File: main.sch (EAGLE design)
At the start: 3 parts

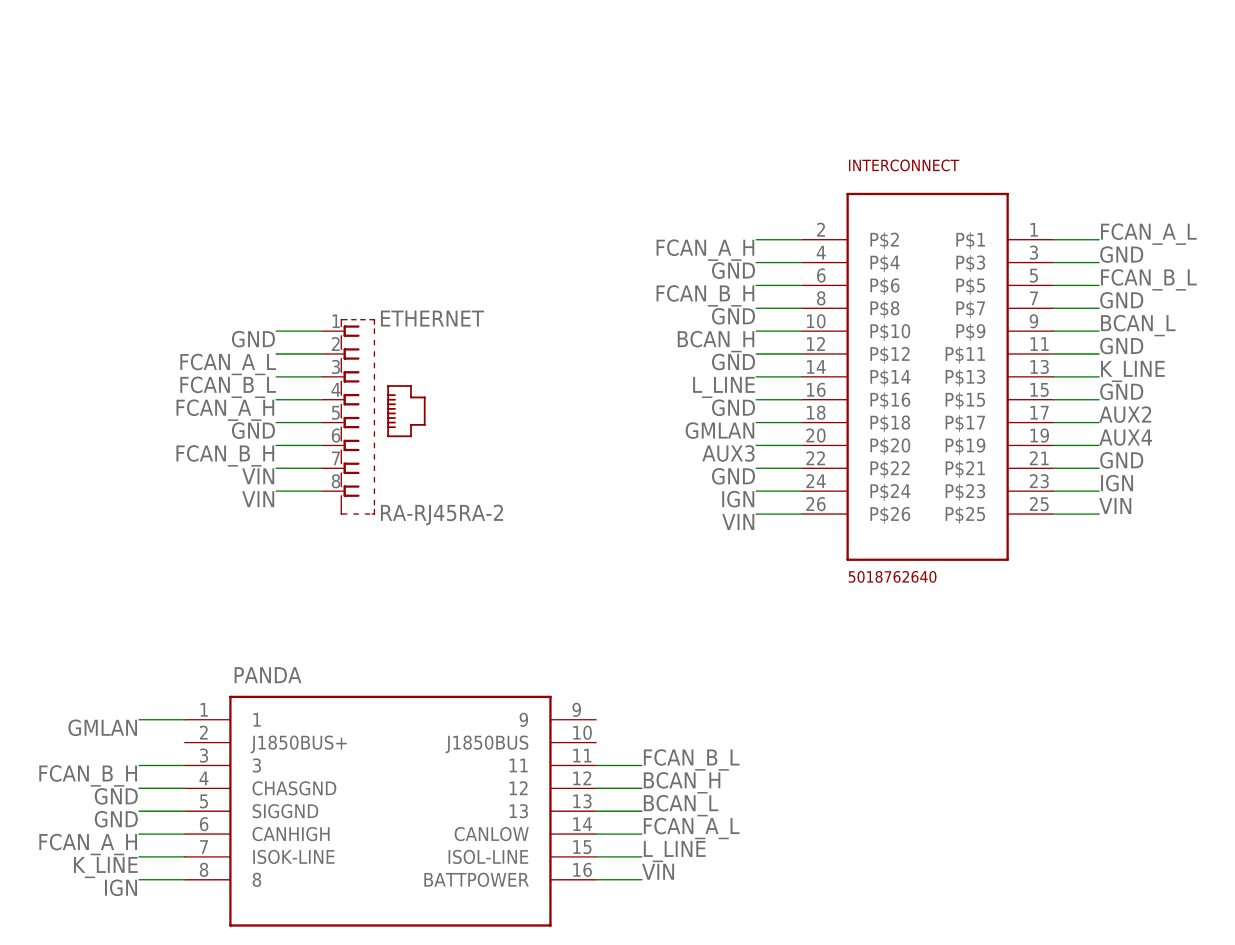
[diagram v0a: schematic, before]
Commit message: push new versions. autorouted!
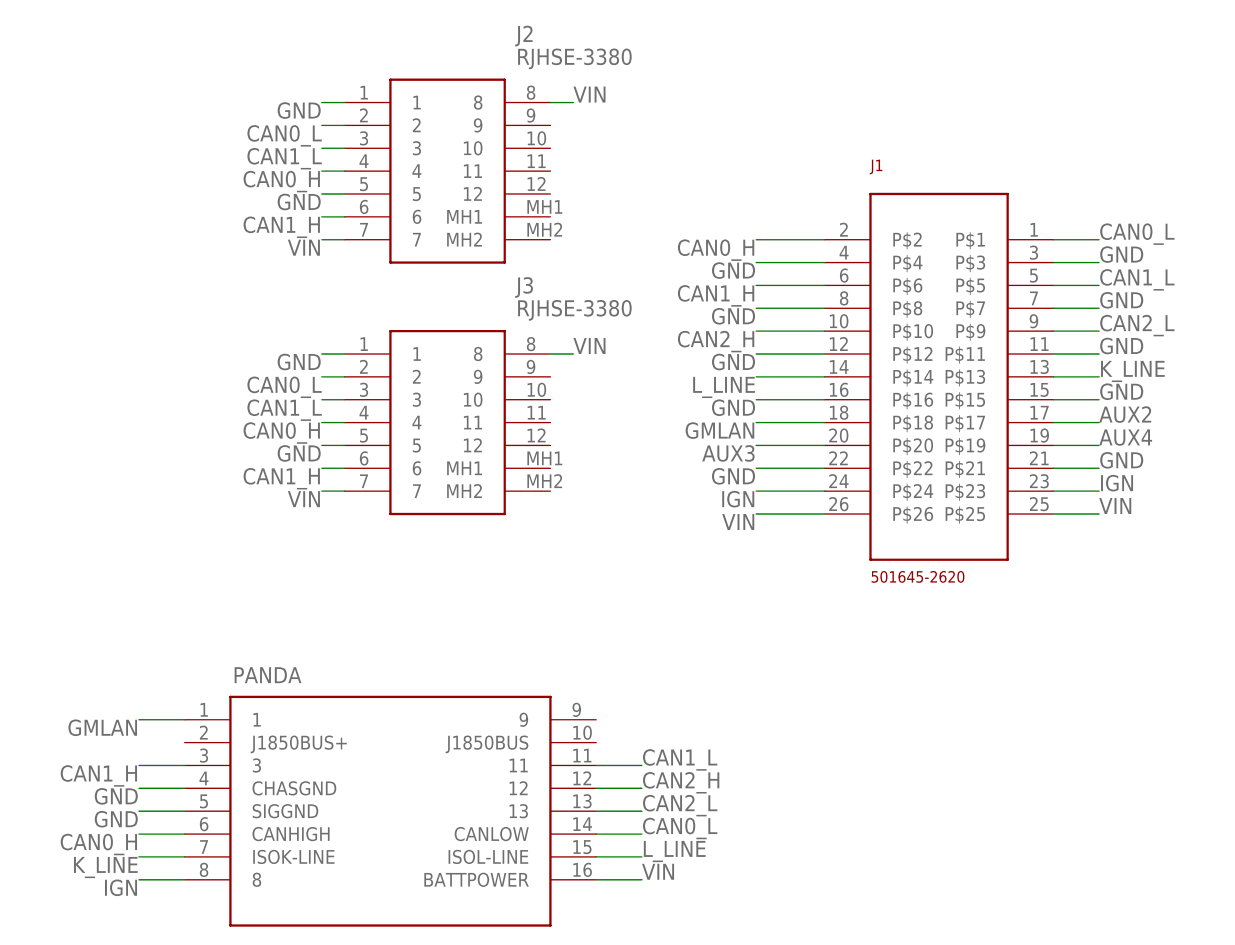
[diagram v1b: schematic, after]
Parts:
- removed ETHERNET: RA-RJ45RA-2, comma.ai:RA-RJ45RA-2
- removed INTERCONNECT: 5018762640, Souers:5018762640
- added J1: 501645-2620, Souers:501645-2620
- added J2, J3: RJHSE-3380, RJHSE-3380:RJHSE-3380
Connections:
- removed net BCAN_H: INTERCONNECT.P$10, PANDA.12
- removed net BCAN_L: INTERCONNECT.P$9, PANDA.13
- removed net FCAN_A_H: ETHERNET.4, INTERCONNECT.P$2, PANDA.CANHIGH
- removed net FCAN_A_L: ETHERNET.2, INTERCONNECT.P$1, PANDA.CANLOW
- removed net FCAN_B_H: ETHERNET.6, INTERCONNECT.P$6, PANDA.3
- removed net FCAN_B_L: ETHERNET.3, INTERCONNECT.P$5, PANDA.11
- new net CAN0_H: J1.P$2, J2.4, J3.4, PANDA.CANHIGH
- new net CAN0_L: J1.P$1, J2.2, J3.2, PANDA.CANLOW
- new net CAN1_H: J1.P$6, J2.6, J3.6, PANDA.3
- new net CAN1_L: J1.P$5, J2.3, J3.3, PANDA.11
- new net CAN2_H: J1.P$10, PANDA.12
- new net CAN2_L: J1.P$9, PANDA.13
- net AUX2: now also J1.P$17; no longer INTERCONNECT.P$17
- net AUX3: now also J1.P$20; no longer INTERCONNECT.P$20
- net AUX4: now also J1.P$19; no longer INTERCONNECT.P$19
- net GMLAN: now also J1.P$18; no longer INTERCONNECT.P$18
- net GND: now also J1.P$11, J1.P$12, J1.P$15, J1.P$16, J1.P$21, J1.P$22, J1.P$3, J1.P$4, J1.P$7, J1.P$8, J2.1, J2.5, J3.1, J3.5; no longer ETHERNET.1, ETHERNET.5, INTERCONNECT.P$11, INTERCONNECT.P$12, INTERCONNECT.P$15, INTERCONNECT.P$16, INTERCONNECT.P$21, INTERCONNECT.P$22, INTERCONNECT.P$3, INTERCONNECT.P$4, INTERCONNECT.P$7, INTERCONNECT.P$8
- net IGN: now also J1.P$23, J1.P$24; no longer INTERCONNECT.P$23, INTERCONNECT.P$24
- net K_LINE: now also J1.P$13; no longer INTERCONNECT.P$13
- net L_LINE: now also J1.P$14; no longer INTERCONNECT.P$14
- net VIN: now also J1.P$25, J1.P$26, J2.7, J2.8, J3.7, J3.8; no longer ETHERNET.7, ETHERNET.8, INTERCONNECT.P$25, INTERCONNECT.P$26
